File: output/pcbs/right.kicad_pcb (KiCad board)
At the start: 2 copper layers, 143.6 x 118.9 mm, 72 parts

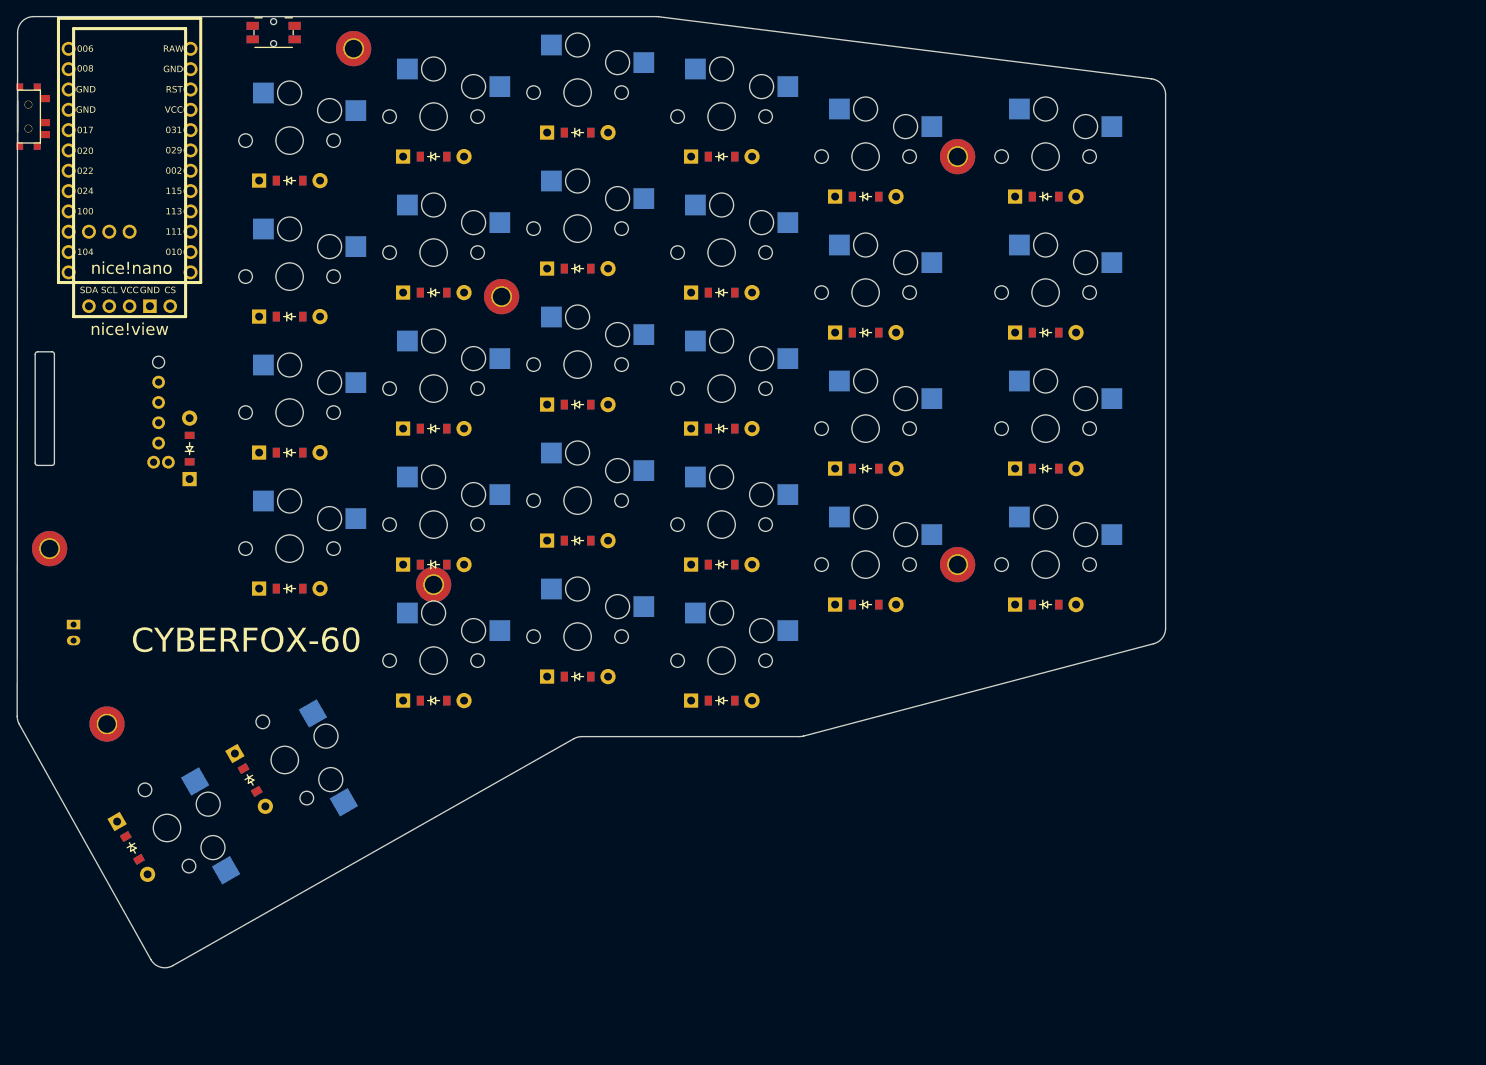
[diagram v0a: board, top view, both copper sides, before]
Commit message: Starting to trace the PCB
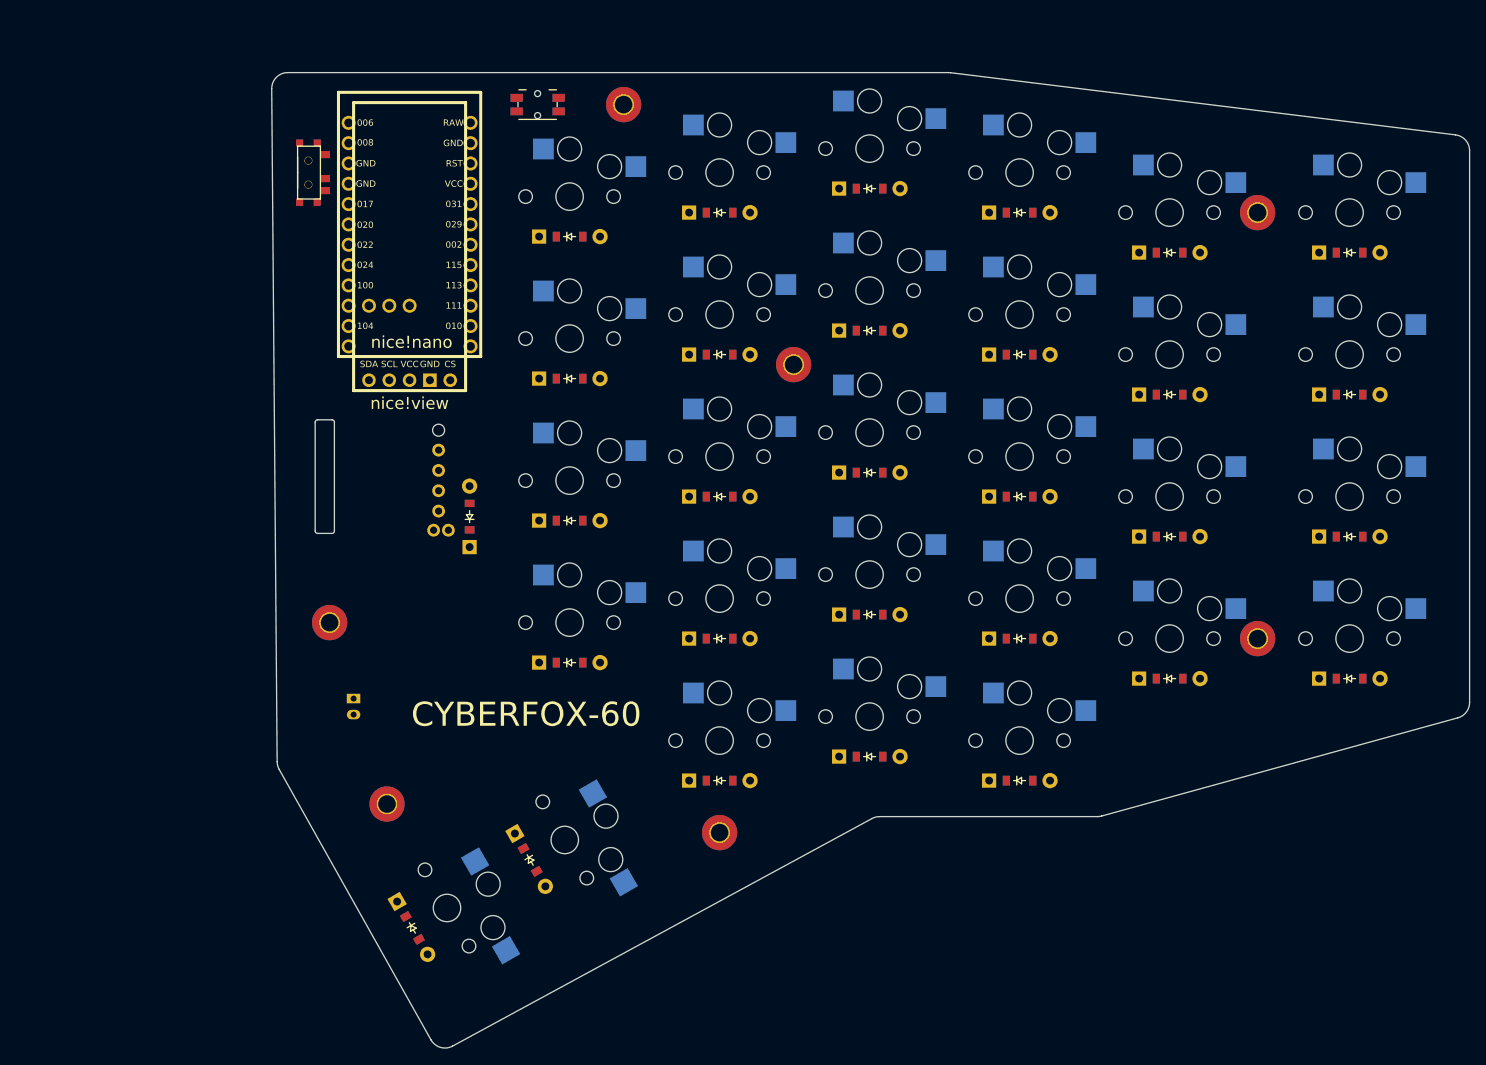
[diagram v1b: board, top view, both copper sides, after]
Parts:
- moved _8 47.3 mm to (231.9, 116.5)
- moved D1 39.1 mm to (310.6, 97.2)
- moved D5 39.1 mm to (288.1, 97.2)
- moved S1 39.1 mm to (310.6, 92.2)
- moved S5 39.1 mm to (288.1, 92.2)
- moved D2 38.9 mm to (310.6, 79.5)
- moved D6 38.9 mm to (288.1, 79.5)
- moved S2 38.9 mm to (310.6, 74.5)
- moved S6 38.9 mm to (288.1, 74.5)
- moved D3 38.8 mm to (310.6, 61.8)
- moved D7 38.8 mm to (288.1, 61.8)
- moved S3 38.8 mm to (310.6, 56.8)
- moved S7 38.8 mm to (288.1, 56.8)
- moved D4 38.6 mm to (310.6, 44.0)
- moved D8 38.6 mm to (288.1, 44.0)
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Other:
- board size 143.6 x 118.9 mm -> 149.7 x 121.9 mm
